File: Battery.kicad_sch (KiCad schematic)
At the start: 6 parts, among them J14 282834-4, J16 282834-2, J17 282834-2

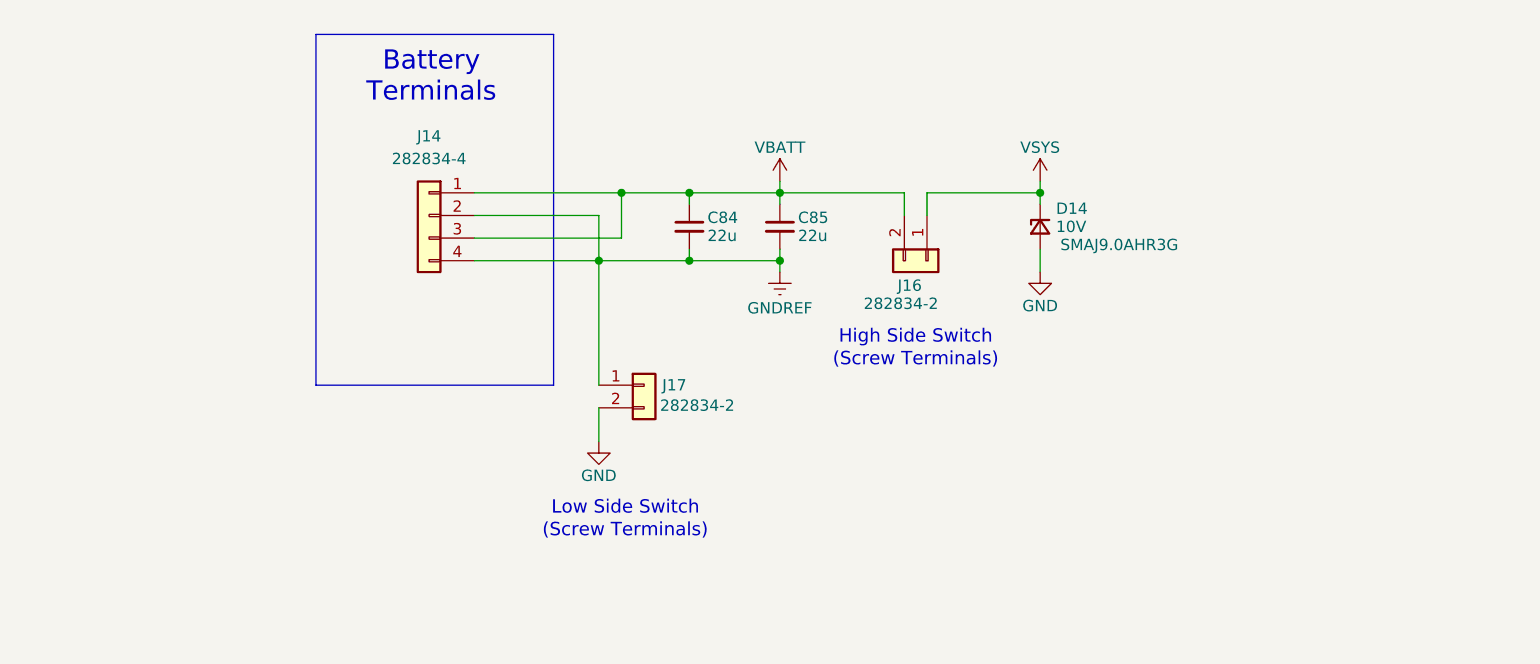
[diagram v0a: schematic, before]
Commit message: v4.0 Updates
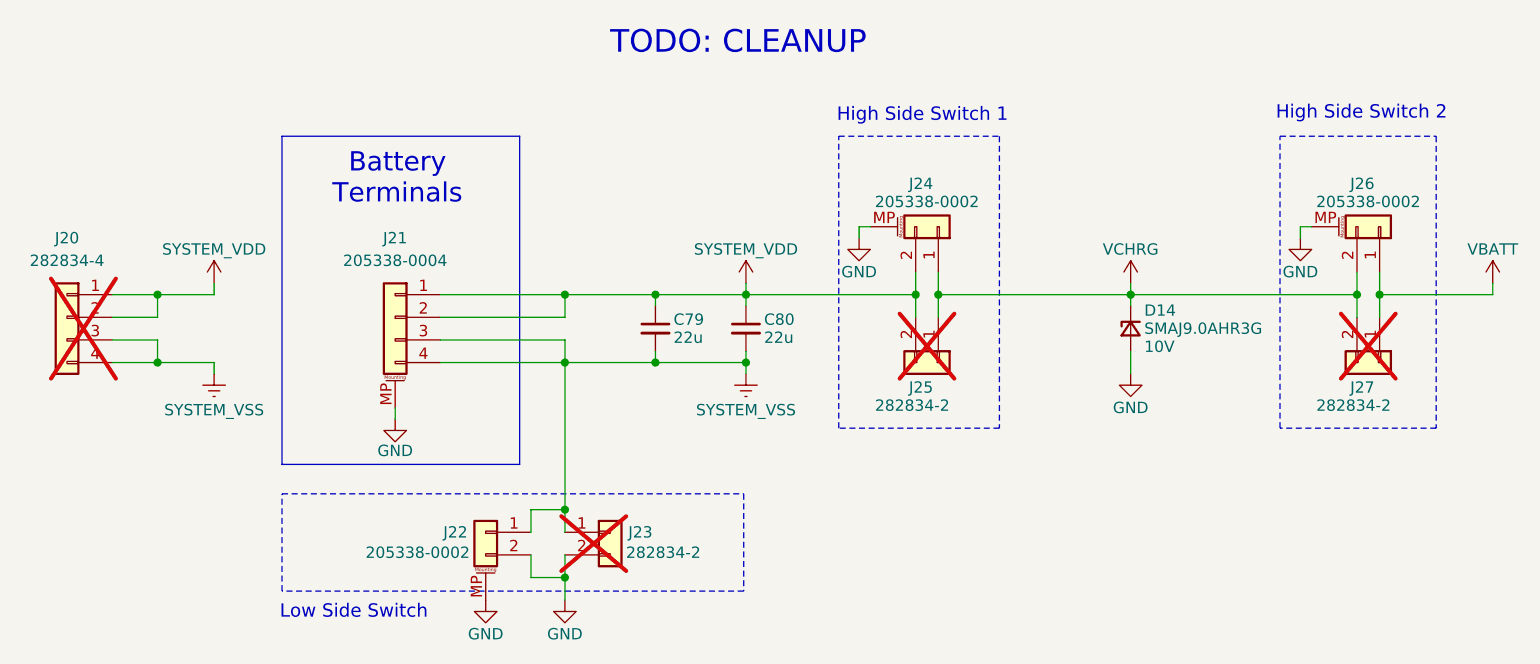
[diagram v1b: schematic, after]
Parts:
- added J21: 205338-0004, Connector_Molex:Molex_Pico-Lock_205338-0004_1x04-1MP_P2.00mm_Horizontal, symbol Connector_Generic_MountingPin:Conn_01x04_MountingPin
- added J22, J24, J26: 205338-0002, Connector_Molex:Molex_Pico-Lock_205338-0002_1x02-1MP_P2.00mm_Horizontal, symbol Connector_Generic_MountingPin:Conn_01x02_MountingPin
- added J27: 282834-2, Argus-Connectors:TE_282834-2, symbol Connector_Generic:Conn_01x02
- D14: value 10V -> SMAJ9.0AHR3G; Part SMAJ9.0AHR3G -> 10V
- J20: renamed from J14; now not fitted
- J23: renamed from J17; now not fitted
- J25: renamed from J16; now not fitted
- renumbered C84 to C79, C85 to C80
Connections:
- net GND: now also J21.MP (MountPin), J22.2 (Pin_2), J22.MP (MountPin), J24.MP (MountPin), J26.MP (MountPin)
- net VBATT: now also J26.1 (Pin_1), J27.1 (Pin_1); no longer C79.1, C80.1, J20.1 (Pin_1), J20.3 (Pin_3), J25.2 (Pin_2)
- net GNDREF renamed SYSTEM_VSS
- net SYSTEM_VSS: now also J20.3 (Pin_3), J21.3 (Pin_3), J21.4 (Pin_4), J22.1 (Pin_1); no longer J20.2 (Pin_2)
- net VSYS renamed VCHRG
- net VCHRG: now also J24.1 (Pin_1), J26.2 (Pin_2), J27.2 (Pin_2)
- new net SYSTEM_VDD: C79.1, C80.1, J20.1 (Pin_1), J20.2 (Pin_2), J21.1 (Pin_1), J21.2 (Pin_2), J24.2 (Pin_2), J25.2 (Pin_2)
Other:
- note added: "High Side Switch 1"
- note added: "High Side Switch 2"
- note added: "TODO: CLEANUP"
- note removed: "(Screw Terminals)"
- note removed: "High Side Switch"
- moved on the sheet: C79, C80, D14

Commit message: DFM updates
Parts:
- C79, C80: MPN (none) -> C2803395
- J20, J23, J25, J27: now left out of the parts list
- J21: MPN (none) -> C916325
- J22, J24, J26: MPN (none) -> C17575002
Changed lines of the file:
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@@
+			)
+		)
+		(property "MPN" "C17575002"
+			(at 229.87 81.28 90)
+			(effects
+				(font
+					(size 1.27 1.27)
+				)
+				(hide yes)
 			)
 		)
@@
 		(unit 1)
 		(exclude_from_sim no)
-		(in_bom yes)
+		(in_bom no)
 		(on_board yes)
 		(dnp yes)
@@
 			)
 		)
+		(property "MPN" "C916325"
+			(at 119.38 91.44 0)
+			(effects
+				(font
+					(size 1.27 1.27)
+				)
+				(hide yes)
+			)
+		)
 		(pin "2"
 		)
@@
 			)
 		)
-		(property "Description" "0.1uF +-10% 50V X7R 0603"
+		(property "Description" ""
+			(at 148.59 92.71 0)
+			(effects
+				(font
+					(size 1.27 1.27)
+				)
+				(hide yes)
+			)
+		)
+		(property "MPN" "C2803395"
 			(at 148.59 92.71 0)
 			(effects
@@
 		(unit 1)
 		(exclude_from_sim no)
-		(in_bom yes)
+		(in_bom no)
 		(on_board yes)
 		(dnp yes)
@@
 		(unit 1)
 		(exclude_from_sim no)
-		(in_bom yes)
+		(in_bom no)
 		(on_board yes)
 		(dnp yes)
@@
 			)
 		)
+		(property "MPN" "C17575002"
+			(at 129.54 115.57 0)
+			(effects
+				(font
+					(size 1.27 1.27)
+				)
+				(hide yes)
+			)
+		)
 		(pin "1"
 		)
@@
 			)
 		)
+		(property "MPN" "C17575002"
+			(at 180.34 81.28 90)
+			(effects
+				(font
+					(size 1.27 1.27)
+				)
+				(hide yes)
+			)
+		)
 		(pin "1"
 		)
@@
 			)
 		)
-		(property "Description" "22uF +-20% 10V X5R"
+		(property "Description" ""
+			(at 158.75 92.71 0)
+			(effects
+				(font
+					(size 1.27 1.27)
+				)
+				(hide yes)
+			)
+		)
+		(property "MPN" "C2803395"
 			(at 158.75 92.71 0)
 			(effects
@@
 		(unit 1)
 		(exclude_from_sim no)
-		(in_bom yes)
+		(in_bom no)
 		(on_board yes)
 		(dnp yes)
